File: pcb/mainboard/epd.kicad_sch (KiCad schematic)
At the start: 13 parts, among them J3 FH12-16S-0.5SH, J4 FH12-50S-0.5SH, J5 FH12-8S-0.5SH

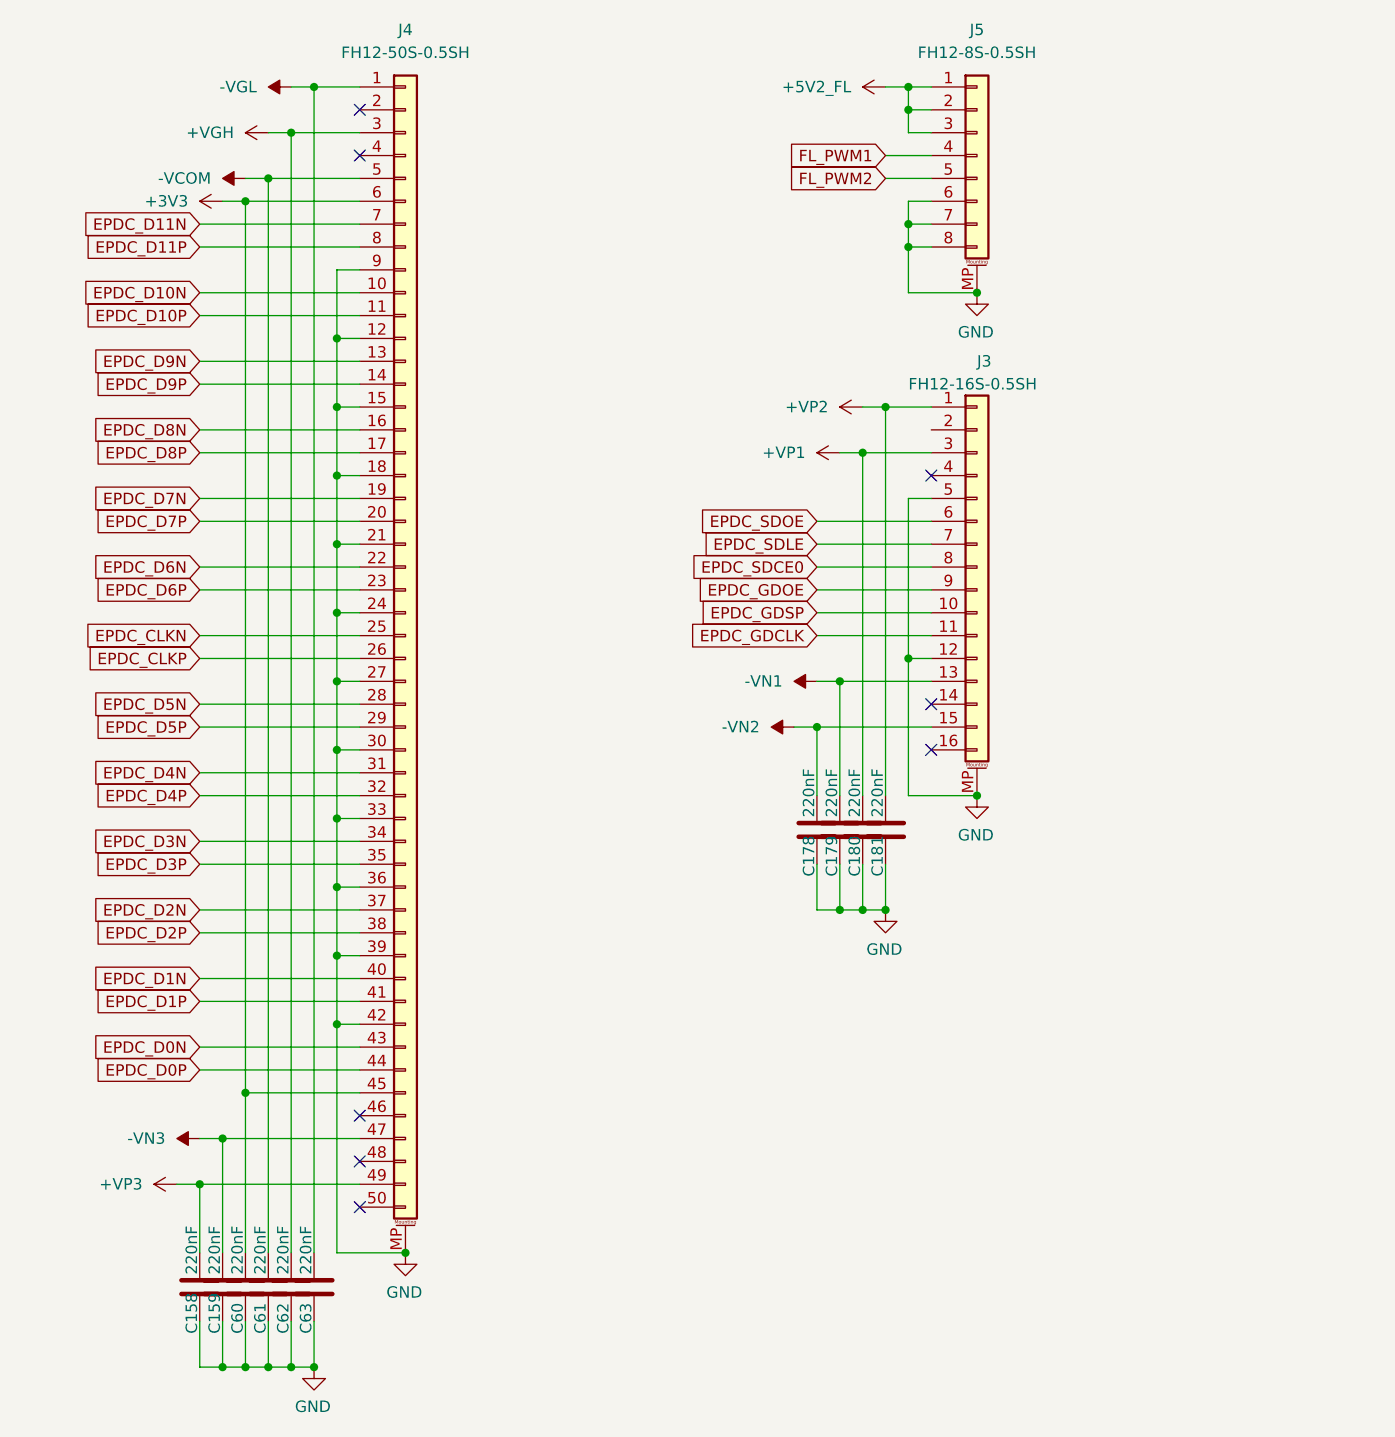
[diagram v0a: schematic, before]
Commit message: PCB r0p10
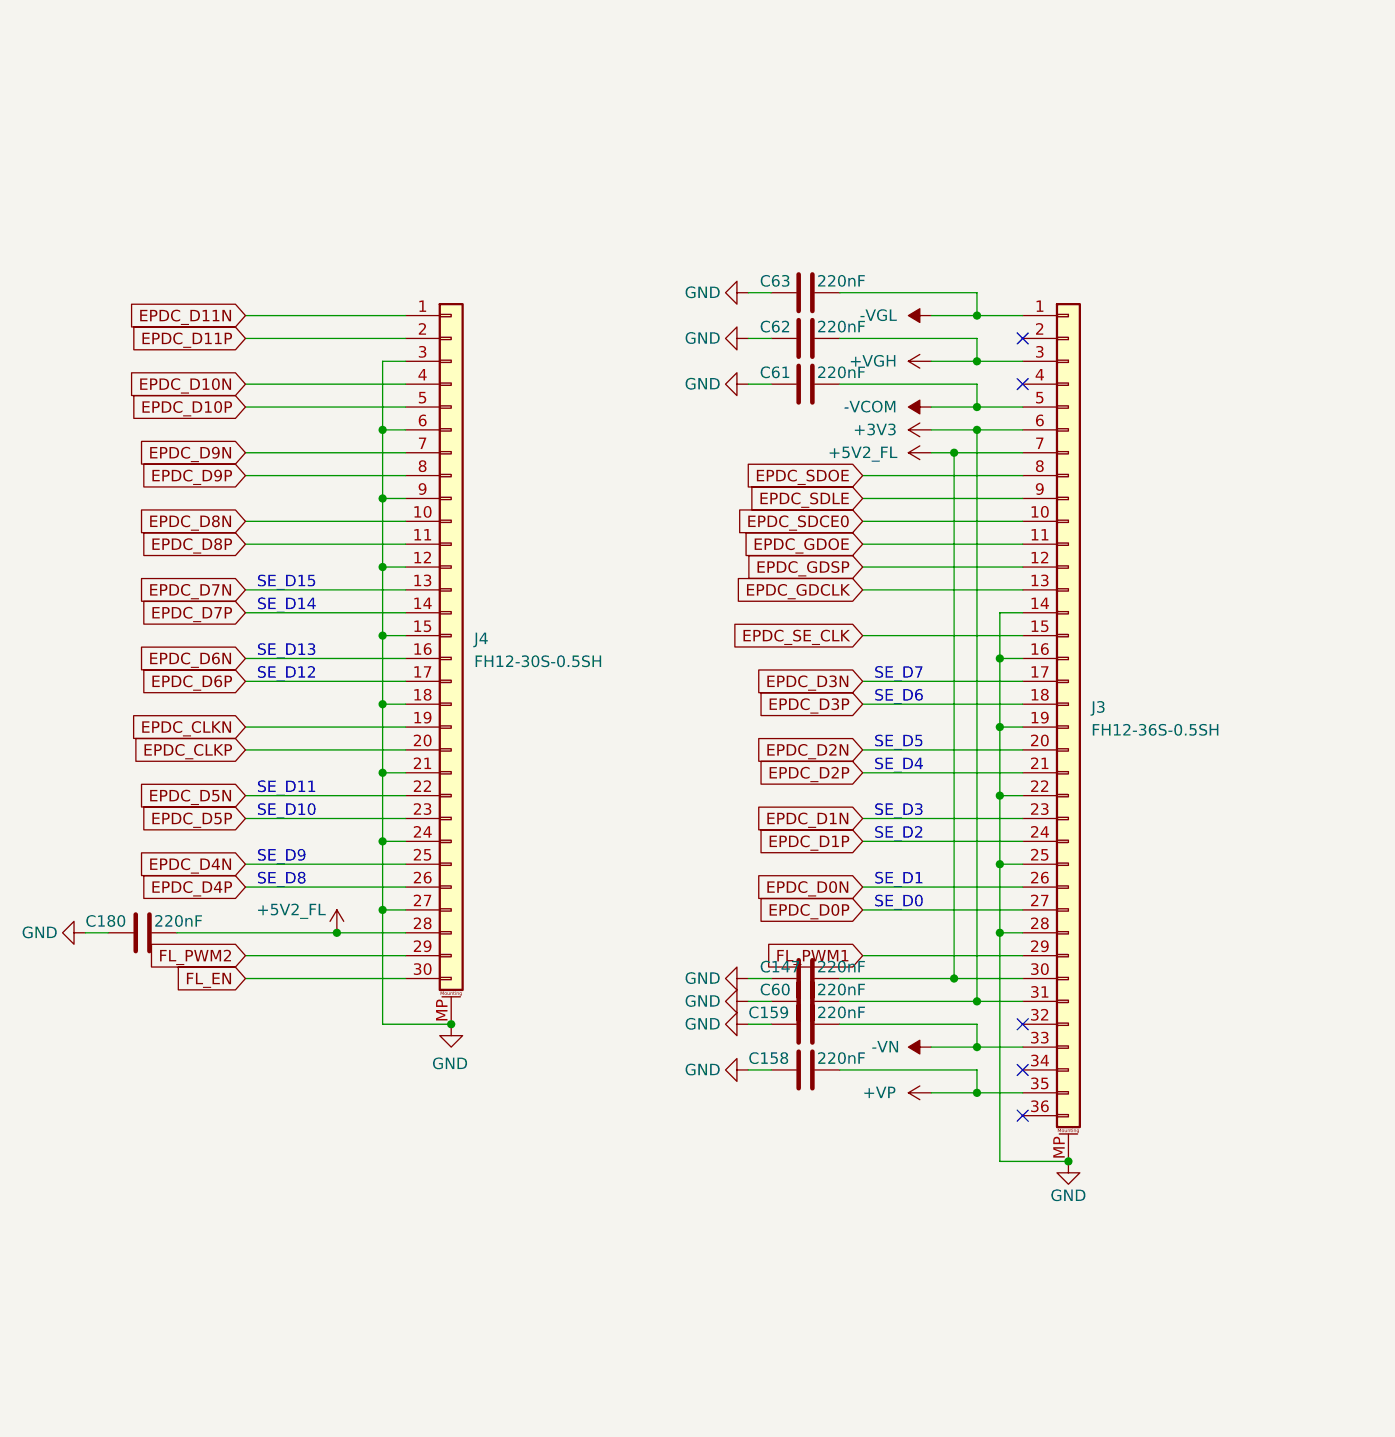
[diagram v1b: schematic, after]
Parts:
- removed C178, C179, C181: 220nF, Capacitor_SMD:C_0402_1005Metric, symbol Device:C
- removed J3: FH12-16S-0.5SH, Connector_FFC-FPC:Hirose_FH12-16S-0.5SH_1x16-1MP_P0.50mm_Horizontal, symbol Connector_Generic_MountingPin:Conn_01x16_MountingPin
- removed J4: FH12-50S-0.5SH, Connector_FFC-FPC:Hirose_FH12-50S-0.5SH_1x50-1MP_P0.50mm_Horizontal, symbol Connector_Generic_MountingPin:Conn_01x50_MountingPin
- removed J5: FH12-8S-0.5SH, Connector_FFC-FPC:Hirose_FH12-8S-0.5SH_1x08-1MP_P0.50mm_Horizontal, symbol Connector_Generic_MountingPin:Conn_01x08_MountingPin
- added C147: 220nF, Capacitor_SMD:C_0402_1005Metric, symbol Device:C
- added J3: FH12-36S-0.5SH, Connector_FFC-FPC:Hirose_FH12-36S-0.5SH_1x36-1MP_P0.50mm_Horizontal, symbol Connector_Generic_MountingPin:Conn_01x36_MountingPin
- added J4: FH12-30S-0.5SH, Connector_FFC-FPC:Hirose_FH12-30S-0.5SH_1x30-1MP_P0.50mm_Horizontal, symbol Connector_Generic_MountingPin:Conn_01x30_MountingPin
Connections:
- net +VP1 is gone; now on net +5V2_FL: C180.1
- net +3V3: now also J3.31 (Pin_31), J3.6 (Pin_6)
- net +5V2_FL: now also C147.1, J3.30 (Pin_30), J3.7 (Pin_7), J4.28 (Pin_28)
- net +VGH: now also J3.3 (Pin_3)
- net -VCOM: now also J3.5 (Pin_5)
- net -VGL: now also J3.1 (Pin_1)
- net EPDC_CLKN: now also J4.19 (Pin_19)
- net EPDC_CLKP: now also J4.20 (Pin_20)
- net EPDC_D0N: now also J3.26 (Pin_26)
- net EPDC_D0P: now also J3.27 (Pin_27)
- net EPDC_D10N: now also J4.4 (Pin_4)
- net EPDC_D10P: now also J4.5 (Pin_5)
- net EPDC_D11N: now also J4.1 (Pin_1)
- net EPDC_D11P: now also J4.2 (Pin_2)
- net EPDC_D1N: now also J3.23 (Pin_23)
- net EPDC_D1P: now also J3.24 (Pin_24)
- net EPDC_D2N: now also J3.20 (Pin_20)
- net EPDC_D2P: now also J3.21 (Pin_21)
- net EPDC_D3N: now also J3.17 (Pin_17)
- net EPDC_D3P: now also J3.18 (Pin_18)
- net EPDC_D4N: now also J4.25 (Pin_25)
- net EPDC_D4P: now also J4.26 (Pin_26)
- net EPDC_D5N: now also J4.22 (Pin_22)
- net EPDC_D5P: now also J4.23 (Pin_23)
- net EPDC_D6N: now also J4.16 (Pin_16)
- net EPDC_D6P: now also J4.17 (Pin_17)
- net EPDC_D7N: now also J4.13 (Pin_13)
- net EPDC_D7P: now also J4.14 (Pin_14)
- net EPDC_D8N: now also J4.10 (Pin_10)
- net EPDC_D8P: now also J4.11 (Pin_11)
- net EPDC_D9N: now also J4.7 (Pin_7)
- net EPDC_D9P: now also J4.8 (Pin_8)
- net EPDC_GDCLK: now also J3.13 (Pin_13)
- net EPDC_GDOE: now also J3.11 (Pin_11)
- net EPDC_GDSP: now also J3.12 (Pin_12)
- net EPDC_SDCE0: now also J3.10 (Pin_10)
- net EPDC_SDLE: now also J3.9 (Pin_9)
- net EPDC_SDOE: now also J3.8 (Pin_8)
- net FL_PWM1: now also J3.29 (Pin_29)
- net FL_PWM2: now also J4.29 (Pin_29)
- net GND: now also C147.2, J3.14 (Pin_14), J3.16 (Pin_16), J3.19 (Pin_19), J3.22 (Pin_22), J3.25 (Pin_25), J3.28 (Pin_28), J3.MP (MountPin), J4.12 (Pin_12), J4.15 (Pin_15), J4.18 (Pin_18), J4.21 (Pin_21), J4.24 (Pin_24), J4.27 (Pin_27), J4.3 (Pin_3), J4.6 (Pin_6), J4.9 (Pin_9), J4.MP (MountPin)
- net +VP3 renamed +VP
- net +VP: now also J3.35 (Pin_35)
- net -VN3 renamed -VN
- net -VN: now also J3.33 (Pin_33)
- new net EPDC_SE_CLK: J3.15 (Pin_15)
- new net FL_EN: J4.30 (Pin_30)
- no-connect marks 8 -> 5
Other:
- note added: "SE_D0"
- note added: "SE_D1"
- note added: "SE_D10"
- note added: "SE_D11"
- note added: "SE_D12"
- note added: "SE_D13"
- note added: "SE_D14"
- note added: "SE_D15"
- note added: "SE_D2"
- note added: "SE_D3"
- note added: "SE_D4"
- note added: "SE_D5"
- note added: "SE_D6"
- note added: "SE_D7"
- note added: "SE_D8"
- note added: "SE_D9"
- moved on the sheet: C158, C159, C180, C60, C61, C62, C63

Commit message: PCB r0p11
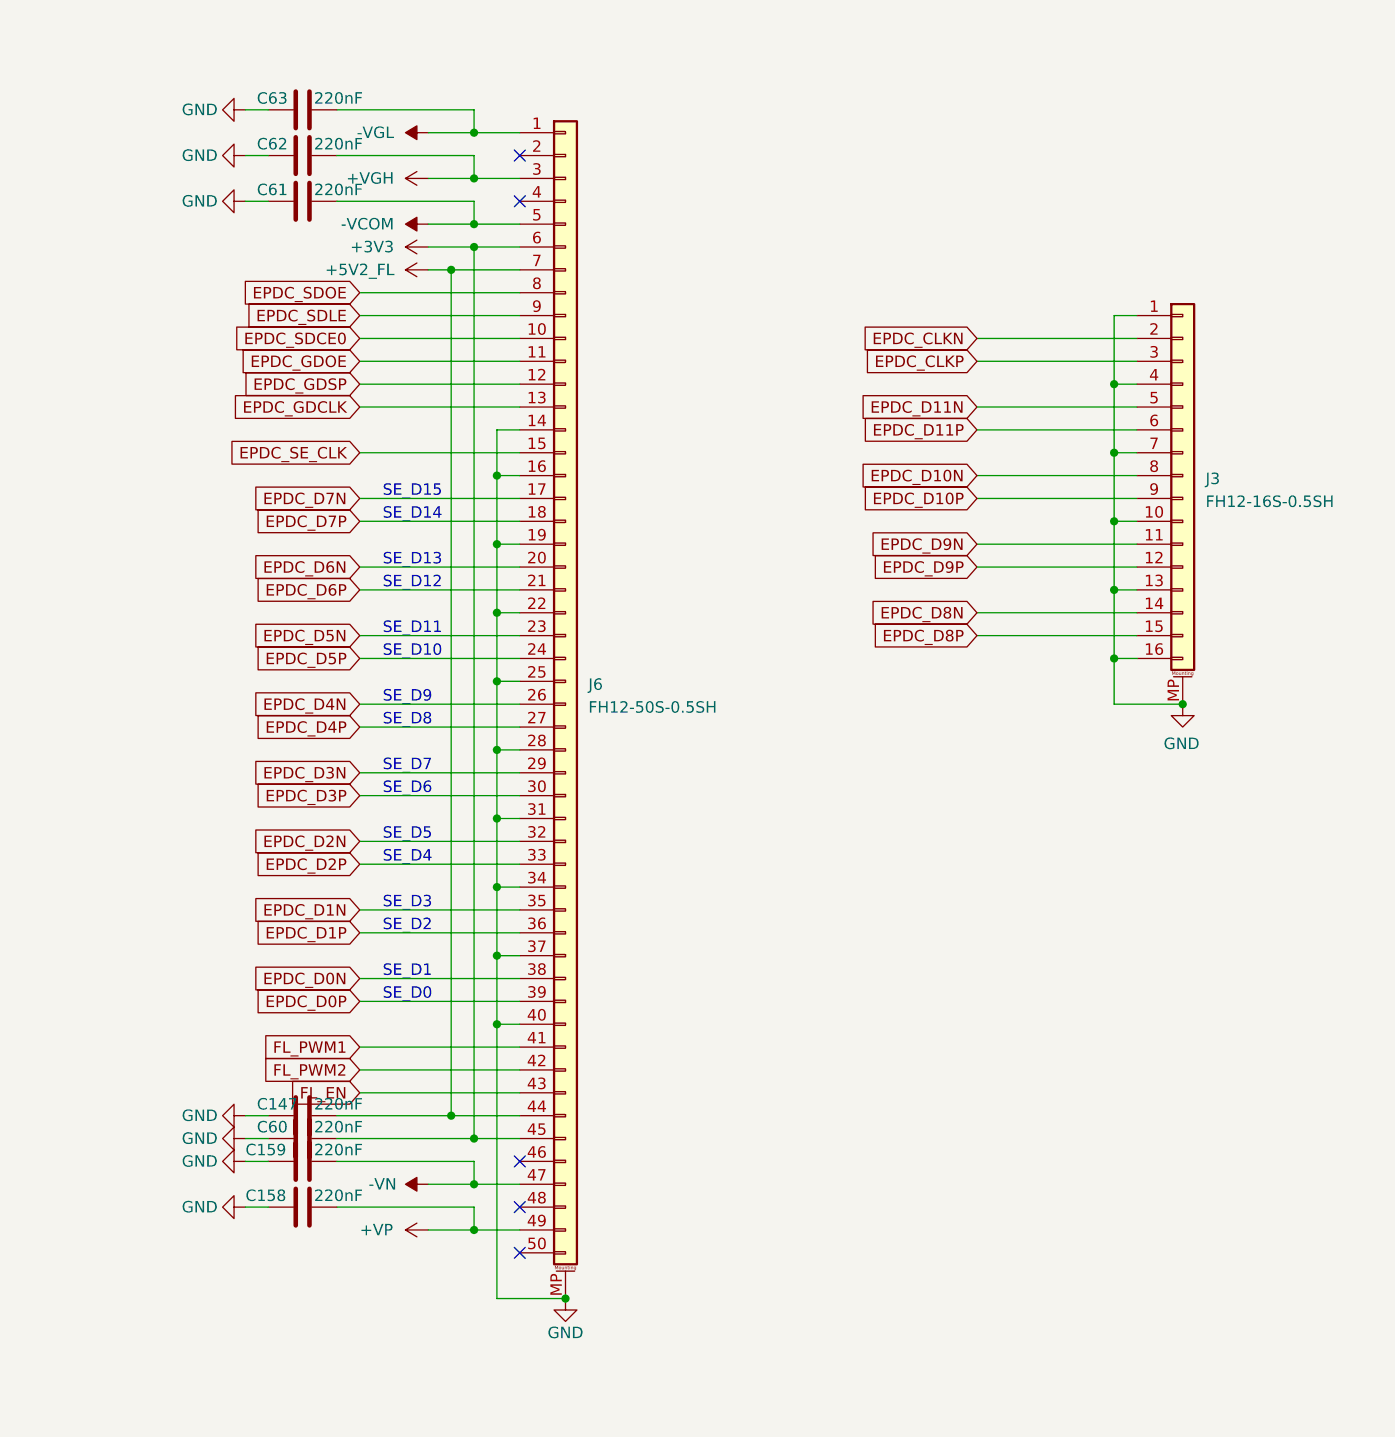
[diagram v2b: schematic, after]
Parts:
- removed C180: 220nF, Capacitor_SMD:C_0402_1005Metric, symbol Device:C
- removed J3: FH12-36S-0.5SH, Connector_FFC-FPC:Hirose_FH12-36S-0.5SH_1x36-1MP_P0.50mm_Horizontal, symbol Connector_Generic_MountingPin:Conn_01x36_MountingPin
- removed J4: FH12-30S-0.5SH, Connector_FFC-FPC:Hirose_FH12-30S-0.5SH_1x30-1MP_P0.50mm_Horizontal, symbol Connector_Generic_MountingPin:Conn_01x30_MountingPin
- added J3: FH12-16S-0.5SH, Connector_FFC-FPC:Hirose_FH12-16S-0.5SH_1x16-1MP_P0.50mm_Horizontal, symbol Connector_Generic_MountingPin:Conn_01x16_MountingPin
- added J6: FH12-50S-0.5SH, Connector_FFC-FPC:Hirose_FH12-50S-0.5SH_1x50-1MP_P0.50mm_Horizontal, symbol Connector_Generic_MountingPin:Conn_01x50_MountingPin
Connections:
- net +3V3: now also J6.45 (Pin_45), J6.6 (Pin_6)
- net +5V2_FL: now also J6.44 (Pin_44), J6.7 (Pin_7)
- net +VGH: now also J6.3 (Pin_3)
- net +VP: now also J6.49 (Pin_49)
- net -VCOM: now also J6.5 (Pin_5)
- net -VGL: now also J6.1 (Pin_1)
- net -VN: now also J6.47 (Pin_47)
- net EPDC_CLKN: now also J3.2 (Pin_2)
- net EPDC_CLKP: now also J3.3 (Pin_3)
- net EPDC_D0N: now also J6.38 (Pin_38)
- net EPDC_D0P: now also J6.39 (Pin_39)
- net EPDC_D10N: now also J3.8 (Pin_8)
- net EPDC_D10P: now also J3.9 (Pin_9)
- net EPDC_D11N: now also J3.5 (Pin_5)
- net EPDC_D11P: now also J3.6 (Pin_6)
- net EPDC_D1N: now also J6.35 (Pin_35)
- net EPDC_D1P: now also J6.36 (Pin_36)
- net EPDC_D2N: now also J6.32 (Pin_32)
- net EPDC_D2P: now also J6.33 (Pin_33)
- net EPDC_D3N: now also J6.29 (Pin_29)
- net EPDC_D3P: now also J6.30 (Pin_30)
- net EPDC_D4N: now also J6.26 (Pin_26)
- net EPDC_D4P: now also J6.27 (Pin_27)
- net EPDC_D5N: now also J6.23 (Pin_23)
- net EPDC_D5P: now also J6.24 (Pin_24)
- net EPDC_D6N: now also J6.20 (Pin_20)
- net EPDC_D6P: now also J6.21 (Pin_21)
- net EPDC_D7N: now also J6.17 (Pin_17)
- net EPDC_D7P: now also J6.18 (Pin_18)
- net EPDC_D8N: now also J3.14 (Pin_14)
- net EPDC_D8P: now also J3.15 (Pin_15)
- net EPDC_D9N: now also J3.11 (Pin_11)
- net EPDC_D9P: now also J3.12 (Pin_12)
- net EPDC_GDCLK: now also J6.13 (Pin_13)
- net EPDC_GDOE: now also J6.11 (Pin_11)
- net EPDC_GDSP: now also J6.12 (Pin_12)
- net EPDC_SDCE0: now also J6.10 (Pin_10)
- net EPDC_SDLE: now also J6.9 (Pin_9)
- net EPDC_SDOE: now also J6.8 (Pin_8)
- net EPDC_SE_CLK: now also J6.15 (Pin_15)
- net FL_EN: now also J6.43 (Pin_43)
- net FL_PWM1: now also J6.41 (Pin_41)
- net FL_PWM2: now also J6.42 (Pin_42)
- net GND: now also J3.1 (Pin_1), J3.10 (Pin_10), J3.13 (Pin_13), J3.16 (Pin_16), J3.4 (Pin_4), J3.7 (Pin_7), J3.MP (MountPin), J6.14 (Pin_14), J6.16 (Pin_16), J6.19 (Pin_19), J6.22 (Pin_22), J6.25 (Pin_25), J6.28 (Pin_28), J6.31 (Pin_31), J6.34 (Pin_34), J6.37 (Pin_37), J6.40 (Pin_40), J6.MP (MountPin)
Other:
- moved on the sheet: C147, C158, C159, C60, C61, C62, C63
